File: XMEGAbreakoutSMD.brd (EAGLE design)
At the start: 160 x 100 mm, 24 parts, among them IC1 XMEGA16A4

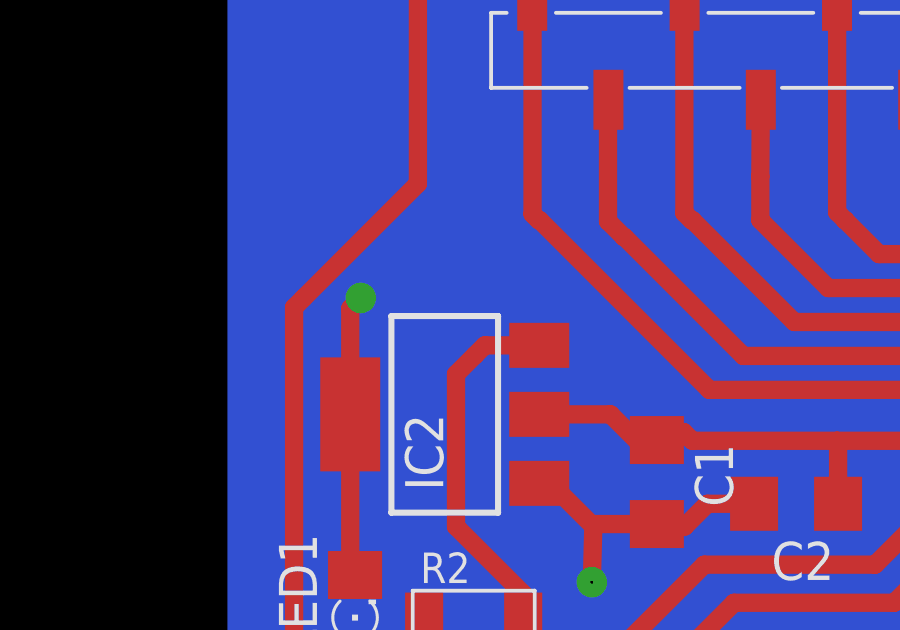
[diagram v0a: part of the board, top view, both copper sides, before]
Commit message: small changes
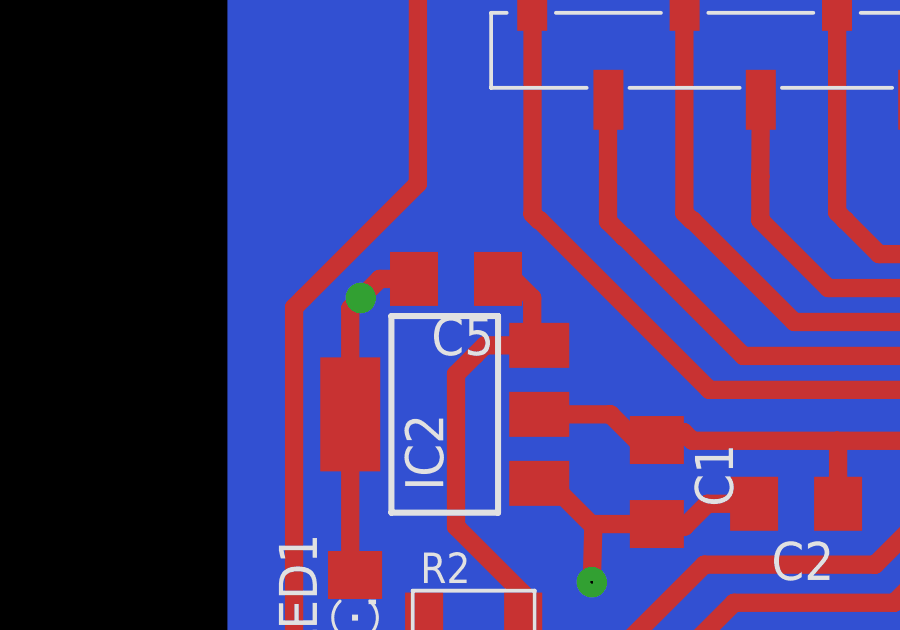
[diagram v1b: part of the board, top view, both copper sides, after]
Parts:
- added C5: 4.7uF, fab:C1206
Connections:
- net GND: now also C5.2
- net VBUS: now also C5.1
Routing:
- net VBUS: track 107.4 -> 110.5 mm
- net GND: track 163.4 -> 165.4 mm
